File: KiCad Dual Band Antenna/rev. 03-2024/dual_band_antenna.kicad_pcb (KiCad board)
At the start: 2 copper layers, 114.4 x 47.1 mm, 5 parts

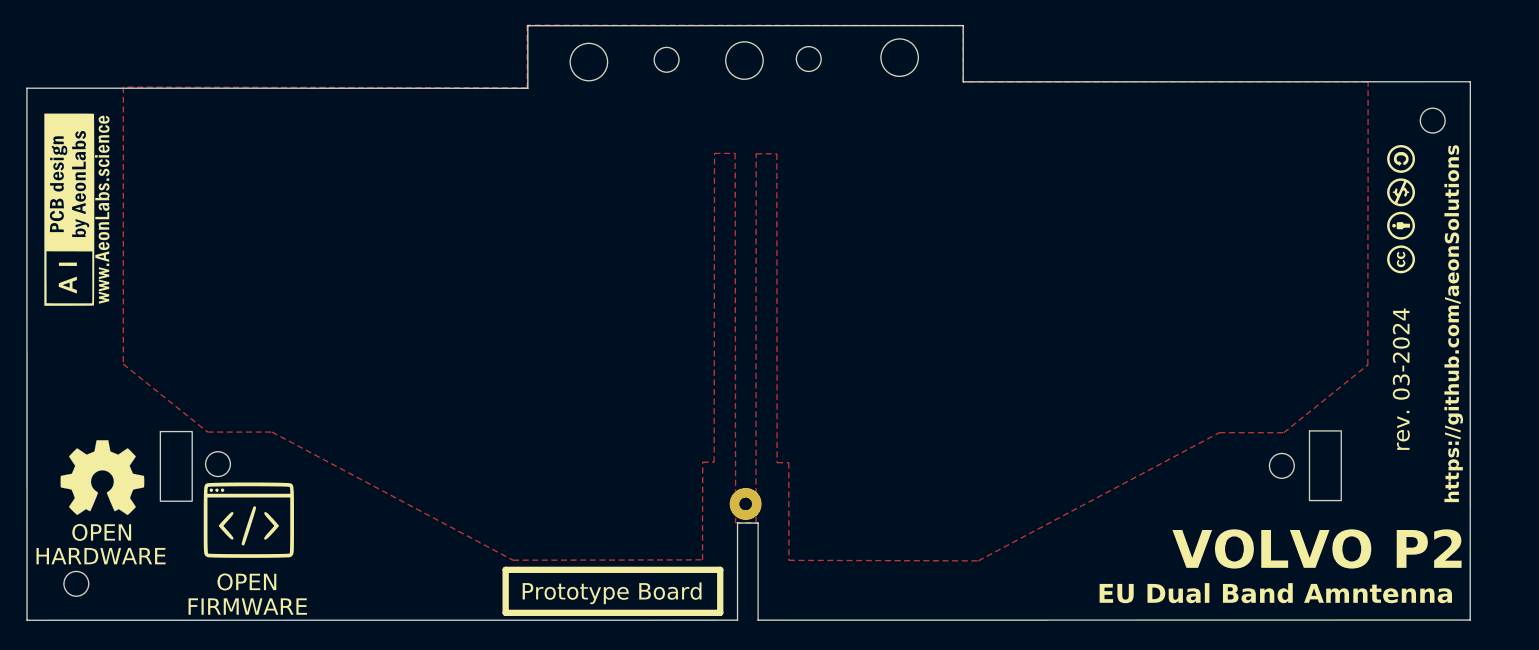
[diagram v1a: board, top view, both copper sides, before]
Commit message: Add files via upload
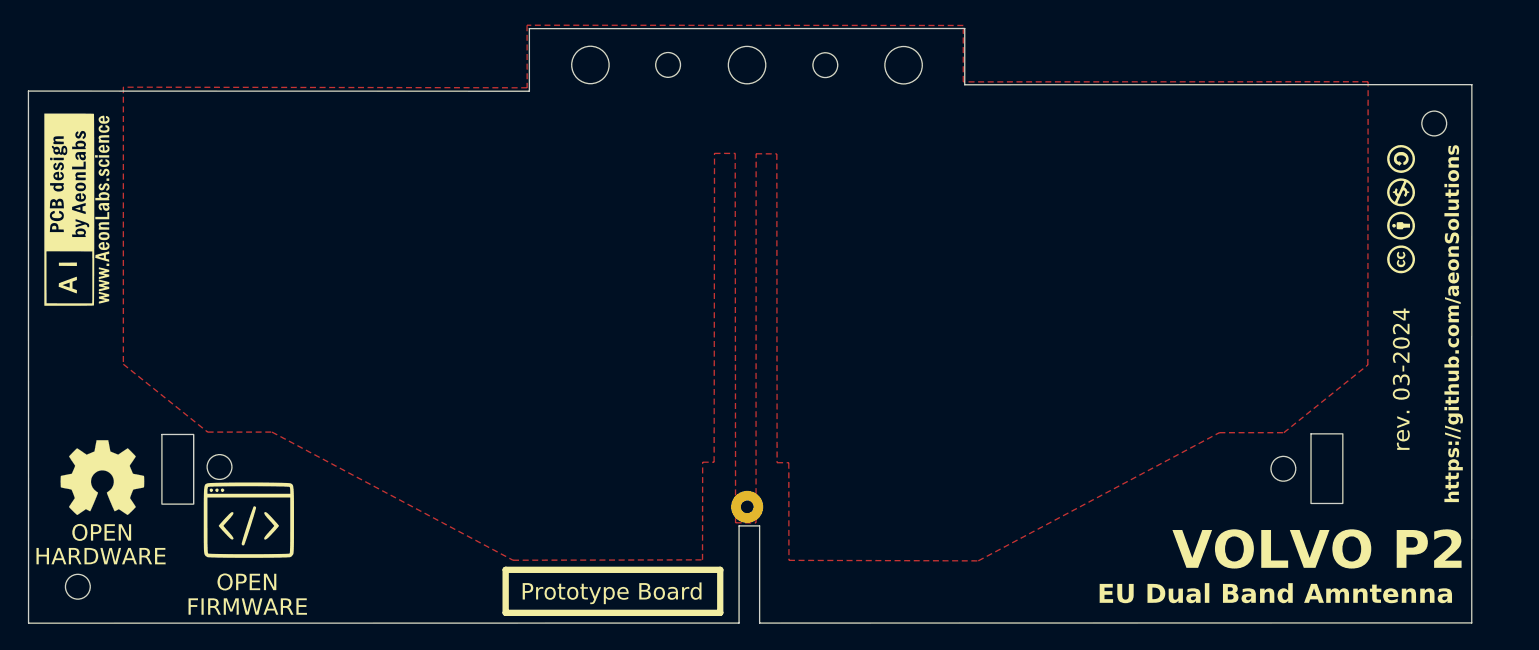
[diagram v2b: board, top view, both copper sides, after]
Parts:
- moved G*** 0.26 mm to (149.7, 97.2)
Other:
- outline, holes or cut-outs redrawn
